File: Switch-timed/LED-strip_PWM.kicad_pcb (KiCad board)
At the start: 2 copper layers, 32 x 16 mm, 17 parts, among them IC1 MADW__ATTINY13-MM, P1 CONN_2, P2 CONN_2, T1 AO3400, U1 MCP6001, U2 MCP1804-SOT23-5

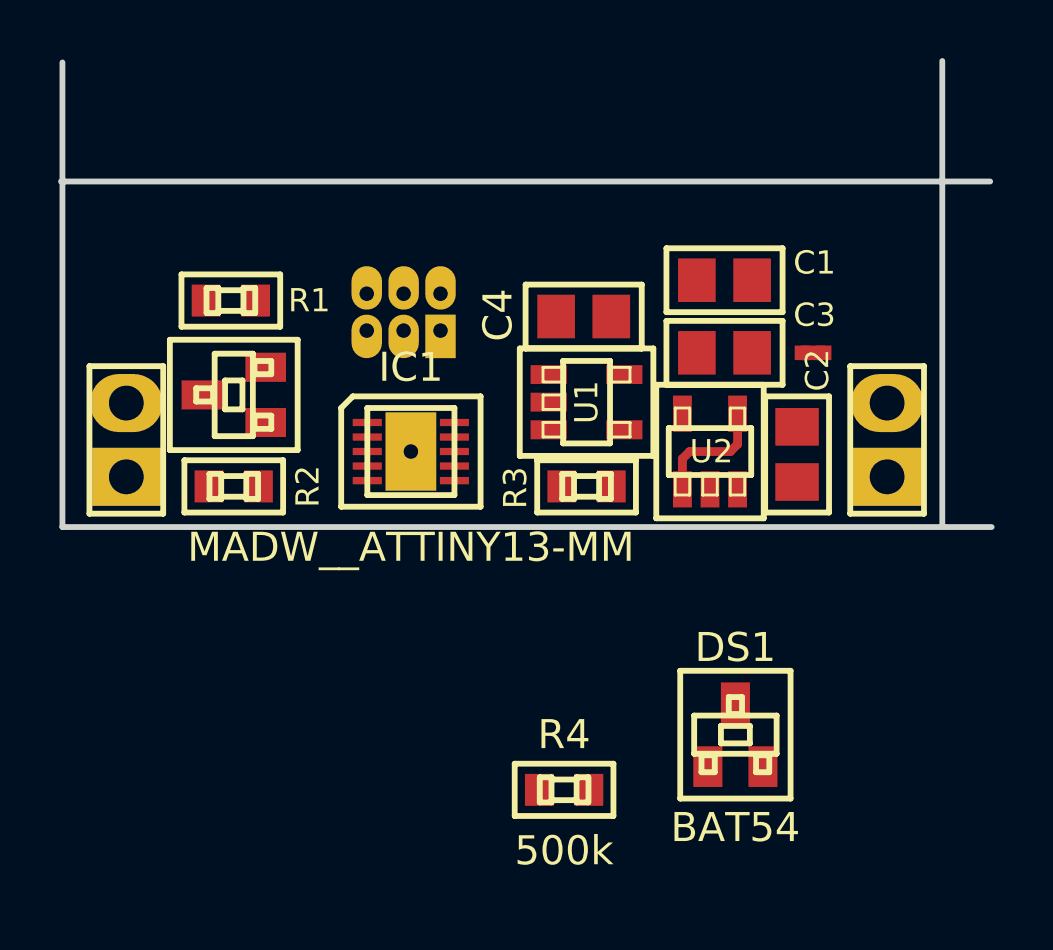
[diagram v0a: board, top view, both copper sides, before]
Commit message: Switch-timed: switched to ATtiny10 SOT23-6.
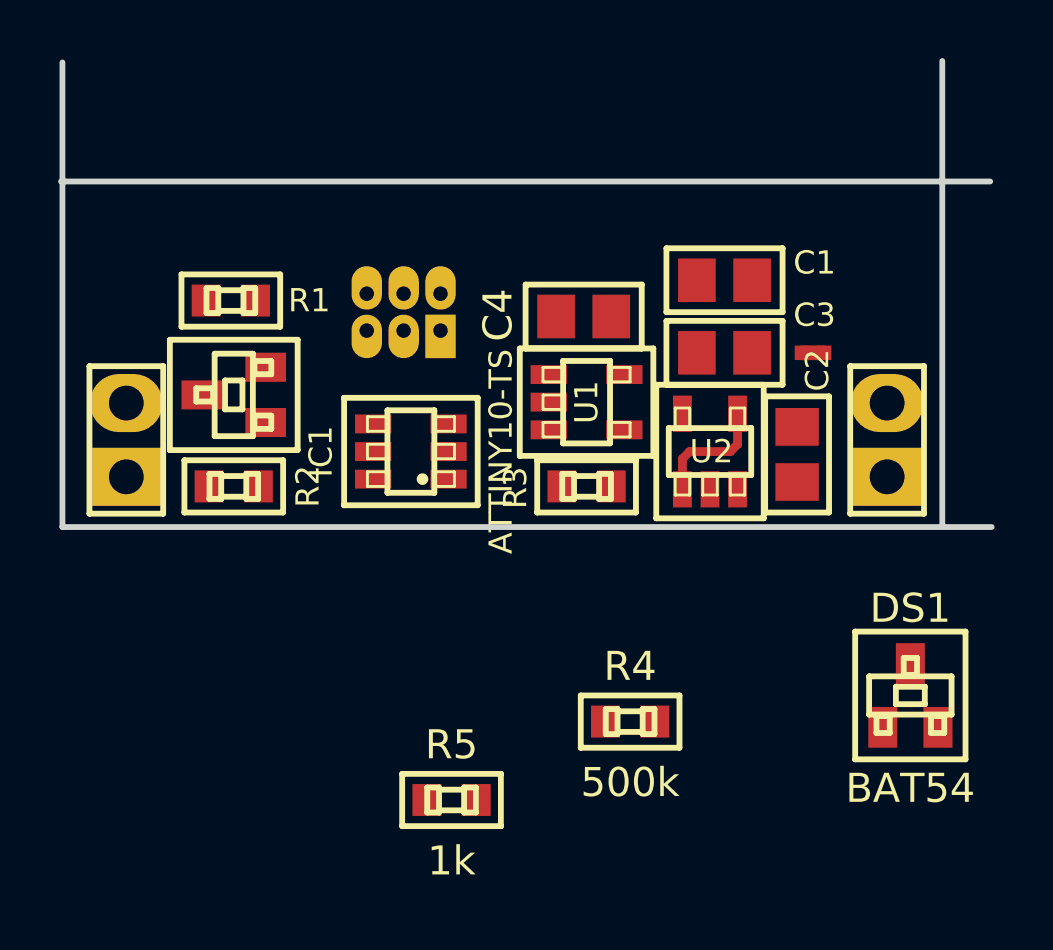
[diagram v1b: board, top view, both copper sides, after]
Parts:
- added R5: 1k, MADW__R0603_2, F.Cu at (89.4, 67.4)
- IC1: value MADW__ATTINY13-MM -> ATTINY10-TS; footprint MADW__MLF10 -> MADW__SOT23-6
- JP1: value ISP -> MADW__AVR_TPI
- R3: value 150R -> 1k
- moved DS1 6.17 mm to (105.2, 63.8)
- moved R4 3.27 mm to (95.5, 64.7)
- turned IC1 to 90 degrees
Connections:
- IC1 pad 1: /RESET -> /GATE
- IC1 pad 2: /SENSE -> GND
- IC1 pad 3: N-000006 -> /SENSE
- IC1 pad 5: GND -> VCC
- IC1 pad 6: /MOSI -> /RESET
- JP1 pad 1: /MISO -> /GATE
- JP1 pad 3: /SCK -> /SENSE
- JP1 pad 4: /MOSI -> N-000007
- R1 pad 2: /MOSI -> /GATE
- R2 pad 1: /MOSI -> /GATE
- U1 pad 1: /SENSE -> N-000002
- U1 pad 4: /SENSE -> N-000002

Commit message: Revert "Switch-timed: switched to ATtiny10 SOT23-6."
This reverts commit 7426c306dc58e77c9809db77e26f6b62b76c1d9c.

C + ATtiny10 not supported by avr-gcc
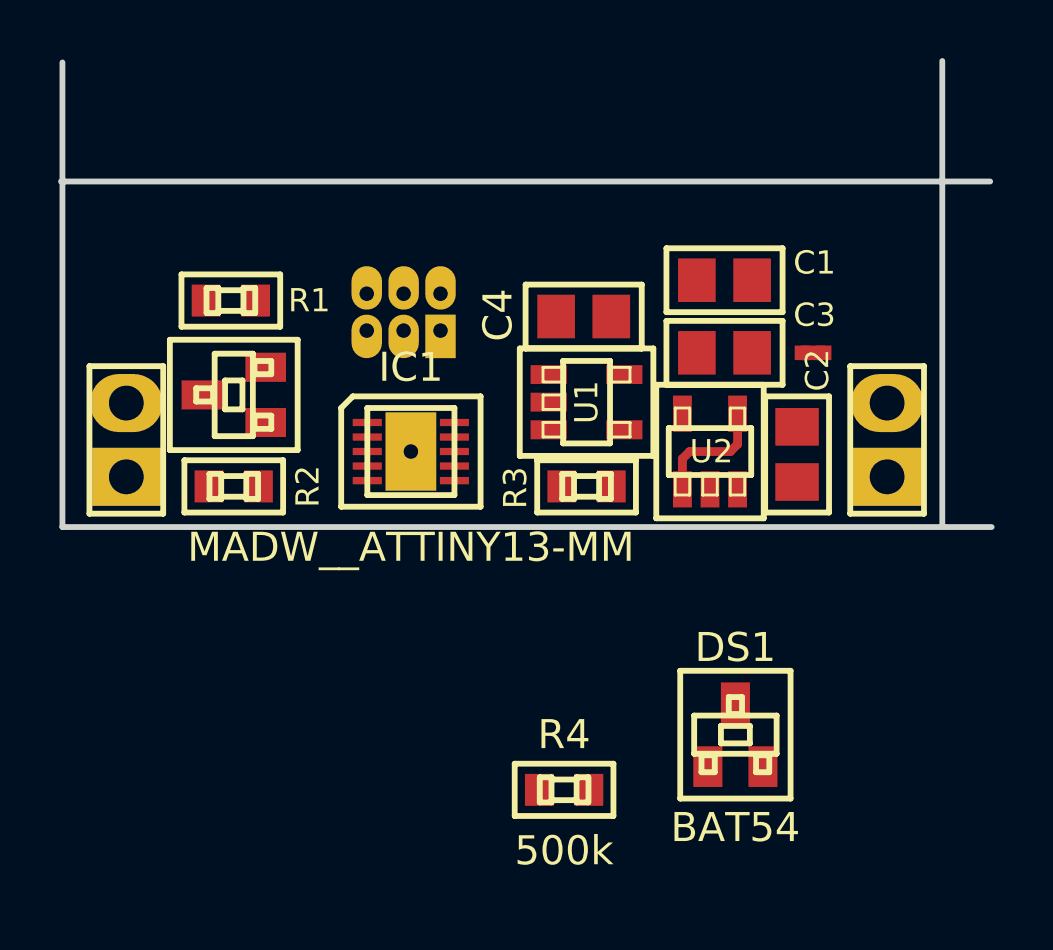
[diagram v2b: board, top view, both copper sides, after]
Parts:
- removed R5: 1k, MADW__R0603_2
- IC1: value ATTINY10-TS -> MADW__ATTINY13-MM; footprint MADW__SOT23-6 -> MADW__MLF10
- JP1: value MADW__AVR_TPI -> ISP
- R3: value 1k -> 150R
- moved DS1 6.17 mm to (99.2, 65.2)
- moved R4 3.27 mm to (93.3, 67.0)
- turned IC1 to 0 degrees
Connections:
- IC1 pad 1: /GATE -> /RESET
- IC1 pad 2: GND -> /SENSE
- IC1 pad 3: /SENSE -> N-000006
- IC1 pad 5: VCC -> GND
- IC1 pad 6: /RESET -> /MOSI
- JP1 pad 1: /GATE -> /MISO
- JP1 pad 3: /SENSE -> /SCK
- JP1 pad 4: N-000007 -> /MOSI
- R1 pad 2: /GATE -> /MOSI
- R2 pad 1: /GATE -> /MOSI
- U1 pad 1: N-000002 (its old number) -> /SENSE
- U1 pad 4: N-000002 (its old number) -> /SENSE
